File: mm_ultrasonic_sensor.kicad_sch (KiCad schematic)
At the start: 0 parts

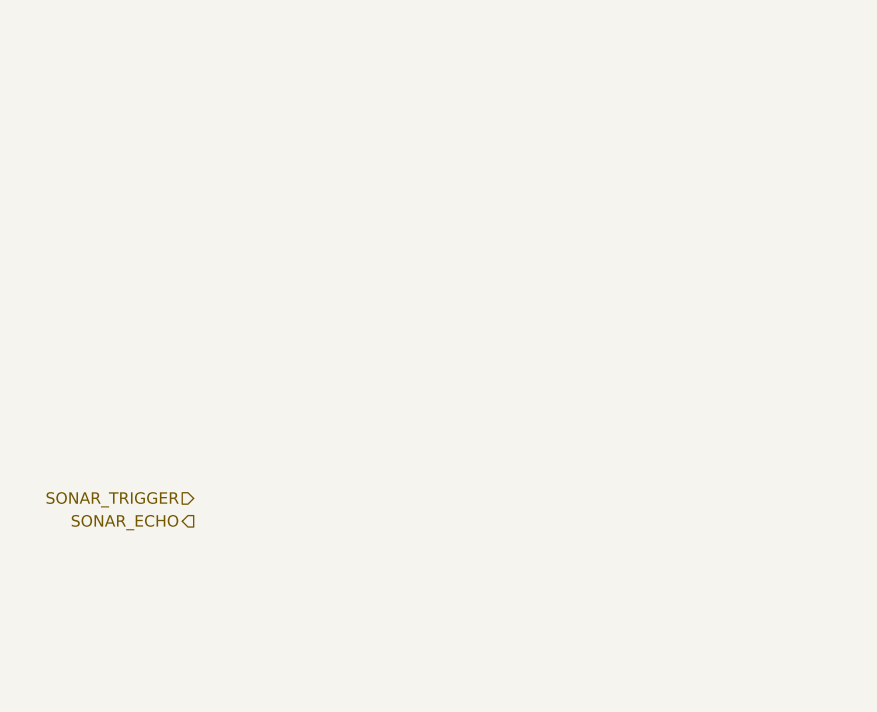
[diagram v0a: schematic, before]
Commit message: tp2
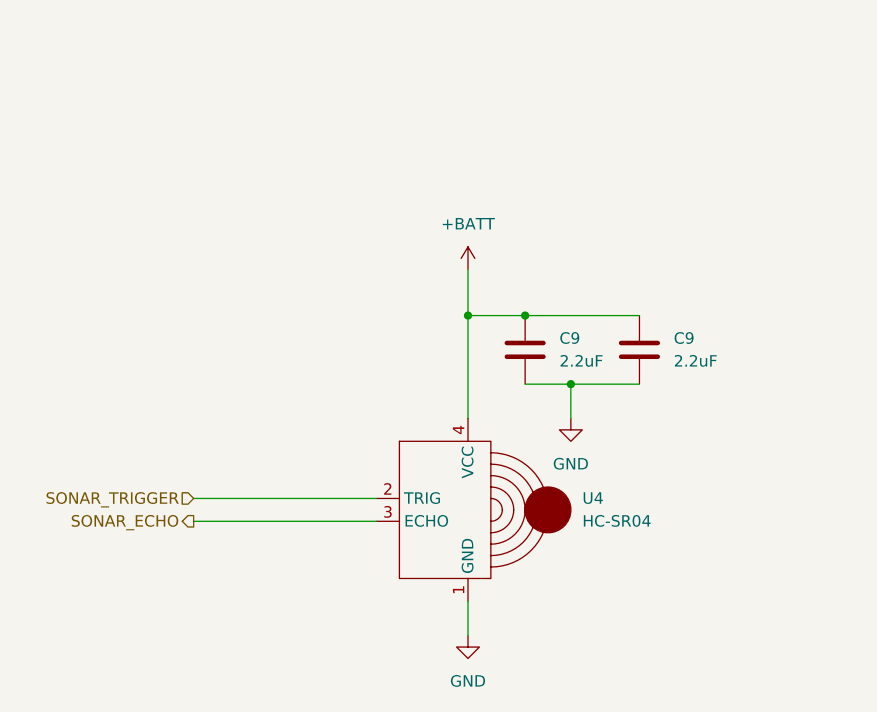
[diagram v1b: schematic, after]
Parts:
- added C9 (x2): 2.2uF, Capacitor_SMD:C_0603_1608Metric, symbol Device:C
- added U4: HC-SR04, minimouse:HC-SR04, symbol minimouse:HC-SR04
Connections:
- net SONAR_ECHO: now also U4.3 (ECHO)
- net SONAR_TRIGGER: now also U4.2 (TRIG)
- new net +BATT: C9.1, C9.1, U4.4 (VCC)
- new net GND: C9.2, C9.2, U4.1 (GND)
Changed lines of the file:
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@@
 (kicad_sch (version 20230121) (generator eeschema)
   (paper "A4")
+  (junction (at 139.7 68.58) (diameter 0) (color 0 0 0 0)
+  )
+  (junction (at 151.13 76.2) (diameter 0) (color 0 0 0 0)
+  )
+  (junction (at 146.05 68.58) (diameter 0) (color 0 0 0 0)
+  )
+  (wire (pts (xy 151.13 76.2) (xy 151.13 80.01))
+    (stroke (width 0) (type default))
+  )
+  (wire (pts (xy 151.13 76.2) (xy 158.75 76.2))
+    (stroke (width 0) (type default))
+  )
+  (wire (pts (xy 139.7 68.58) (xy 146.05 68.58))
+    (stroke (width 0) (type default))
+  )
+  (wire (pts (xy 146.05 76.2) (xy 151.13 76.2))
+    (stroke (width 0) (type default))
+  )
+  (wire (pts (xy 109.22 88.9) (xy 129.54 88.9))
+    (stroke (width 0) (type default))
+  )
+  (wire (pts (xy 139.7 100.33) (xy 139.7 104.14))
+    (stroke (width 0) (type default))
+  )
+  (wire (pts (xy 146.05 68.58) (xy 158.75 68.58))
+    (stroke (width 0) (type default))
+  )
+  (wire (pts (xy 139.7 68.58) (xy 139.7 80.01))
+    (stroke (width 0) (type default))
+  )
+  (wire (pts (xy 139.7 63.5) (xy 139.7 68.58))
+    (stroke (width 0) (type default))
+  )
+  (wire (pts (xy 109.22 91.44) (xy 129.54 91.44))
+    (stroke (width 0) (type default))
+  )
   (hierarchical_label "SONAR_TRIGGER" (shape input) (at 109.22 88.9 180) (fields_autoplaced)
     (effects (font (size 1.27 1.27)) (justify right))
@@
     (effects (font (size 1.27 1.27)) (justify right))
   )
+  (symbol (lib_id "power:GND") (at 151.13 80.01 0) (unit 1)
+    (in_bom yes) (on_board yes) (dnp no) (fields_autoplaced)
+    (property "Reference" "#PWR040" (at 151.13 86.36 0)
+      (effects (font (size 1.27 1.27)) hide)
+    )
+    (property "Value" "GND" (at 151.13 85.09 0)
+      (effects (font (size 1.27 1.27)))
+    )
+    (property "Footprint" "" (at 151.13 80.01 0)
+      (effects (font (size 1.27 1.27)) hide)
+    )
+    (property "Datasheet" "" (at 151.13 80.01 0)
+      (effects (font (size 1.27 1.27)) hide)
+    )
+    (pin "1")
+    (instances
+      (project "minimouse"
+        (path "/d8fa4cba-2469-4231-847f-065b6b829f44/224298a9-7d6e-4a70-a0a5-f2614895ec28"
+          (reference "#PWR040") (unit 1)
+        )
+      )
+    )
+  )
+  (symbol (lib_id "Device:C") (at 158.75 72.39 0) (unit 1)
+    (in_bom yes) (on_board yes) (dnp no) (fields_autoplaced)
+    (property "Reference" "C9" (at 162.56 71.12 0)
+      (effects (font (size 1.27 1.27)) (justify left))
+    )
+    (property "Value" "2.2uF" (at 162.56 73.66 0)
+      (effects (font (size 1.27 1.27)) (justify left))
+    )
+    (property "Footprint" "Capacitor_SMD:C_0603_1608Metric" (at 159.7152 76.2 0)
+      (effects (font (size 1.27 1.27)) hide)
+    )
+    (property "Datasheet" "~" (at 158.75 72.39 0)
+      (effects (font (size 1.27 1.27)) hide)
+    )
+    (pin "1")
+    (pin "2")
+    (instances
+      (project "minimouse"
+        (path "/d8fa4cba-2469-4231-847f-065b6b829f44/d17bb1c7-f68a-465e-9a17-5858ef86fc30"
+          (reference "C9") (unit 1)
+        )
+        (path "/d8fa4cba-2469-4231-847f-065b6b829f44/224298a9-7d6e-4a70-a0a5-f2614895ec28"
+          (reference "C16") (unit 1)
+        )
+      )
+    )
+  )
+  (symbol (lib_id "minimouse:HC-SR04") (at 139.7 90.17 0) (unit 1)
+    (in_bom yes) (on_board yes) (dnp no) (fields_autoplaced)
+    (property "Reference" "U4" (at 152.4 88.9 0)
+      (effects (font (size 1.27 1.27)) (justify left))
+    )
+    (property "Value" "HC-SR04" (at 152.4 91.44 0)
+      (effects (font (size 1.27 1.27)) (justify left))
+    )
+    (property "Footprint" "minimouse:HC-SR04" (at 139.7 90.17 0)
+      (effects (font (size 1.27 1.27)) hide)
+    )
+    (property "Datasheet" "" (at 139.7 90.17 0)
+      (effects (font (size 1.27 1.27)) hide)
+    )
+    (pin "2")
+    (pin "3")
+    (pin "4")
+    (pin "1")
+    (instances
+      (project "minimouse"
+        (path "/d8fa4cba-2469-4231-847f-065b6b829f44/224298a9-7d6e-4a70-a0a5-f2614895ec28"
+          (reference "U4") (unit 1)
+        )
+      )
+    )
+  )
+  (symbol (lib_id "power:+BATT") (at 139.7 63.5 0) (unit 1)
+    (in_bom yes) (on_board yes) (dnp no) (fields_autoplaced)
+    (property "Reference" "#PWR033" (at 139.7 67.31 0)
+      (effects (font (size 1.27 1.27)) hide)
+    )
+    (property "Value" "+BATT" (at 139.7 58.42 0)
+      (effects (font (size 1.27 1.27)))
+    )
+    (property "Footprint" "" (at 139.7 63.5 0)
+      (effects (font (size 1.27 1.27)) hide)
+    )
+    (property "Datasheet" "" (at 139.7 63.5 0)
+      (effects (font (size 1.27 1.27)) hide)
+    )
+    (pin "1")
+    (instances
+      (project "minimouse"
+        (path "/d8fa4cba-2469-4231-847f-065b6b829f44/224298a9-7d6e-4a70-a0a5-f2614895ec28"
+          (reference "#PWR033") (unit 1)
+        )
+      )
+    )
+  )
+  (symbol (lib_id "power:GND") (at 139.7 104.14 0) (unit 1)
+    (in_bom yes) (on_board yes) (dnp no) (fields_autoplaced)
+    (property "Reference" "#PWR032" (at 139.7 110.49 0)
+      (effects (font (size 1.27 1.27)) hide)
+    )
+    (property "Value" "GND" (at 139.7 109.22 0)
+      (effects (font (size 1.27 1.27)))
+    )
+    (property "Footprint" "" (at 139.7 104.14 0)
+      (effects (font (size 1.27 1.27)) hide)
+    )
+    (property "Datasheet" "" (at 139.7 104.14 0)
+      (effects (font (size 1.27 1.27)) hide)
+    )
+    (pin "1")
+    (instances
+      (project "minimouse"
+        (path "/d8fa4cba-2469-4231-847f-065b6b829f44/224298a9-7d6e-4a70-a0a5-f2614895ec28"
+          (reference "#PWR032") (unit 1)
+        )
+      )
+    )
+  )
+  (symbol (lib_id "Device:C") (at 146.05 72.39 0) (unit 1)
+    (in_bom yes) (on_board yes) (dnp no) (fields_autoplaced)
+    (property "Reference" "C9" (at 149.86 71.12 0)
+      (effects (font (size 1.27 1.27)) (justify left))
+    )
+    (property "Value" "2.2uF" (at 149.86 73.66 0)
+      (effects (font (size 1.27 1.27)) (justify left))
+    )
+    (property "Footprint" "Capacitor_SMD:C_0603_1608Metric" (at 147.0152 76.2 0)
+      (effects (font (size 1.27 1.27)) hide)
+    )
+    (property "Datasheet" "~" (at 146.05 72.39 0)
+      (effects (font (size 1.27 1.27)) hide)
+    )
+    (pin "1")
+    (pin "2")
+    (instances
+      (project "minimouse"
+        (path "/d8fa4cba-2469-4231-847f-065b6b829f44/d17bb1c7-f68a-465e-9a17-5858ef86fc30"
+          (reference "C9") (unit 1)
+        )
+        (path "/d8fa4cba-2469-4231-847f-065b6b829f44/224298a9-7d6e-4a70-a0a5-f2614895ec28"
+          (reference "C15") (unit 1)
+        )
+      )
+    )
+  )
 )

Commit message: TP3
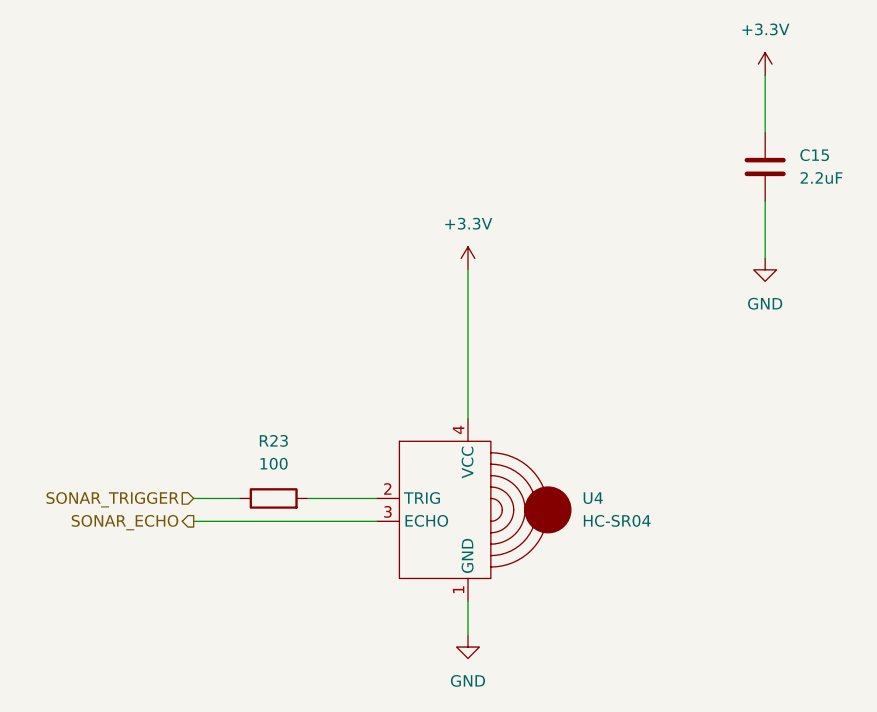
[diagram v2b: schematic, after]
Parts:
- removed C9 (x2): 2.2uF, Capacitor_SMD:C_0603_1608Metric, symbol Device:C
- added C15: 2.2uF, Capacitor_SMD:C_0603_1608Metric, symbol Device:C
- added R23: 100, Resistor_SMD:R_0603_1608Metric, symbol Device:R
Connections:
- net GND: now also C15.2
- net SONAR_TRIGGER: now also R23.1; no longer U4.2 (TRIG)
- net +BATT renamed +3.3V
- net +3.3V: now also C15.1
- new net: R23.2, U4.2 (TRIG)
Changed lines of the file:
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@@
 (kicad_sch (version 20230121) (generator eeschema)
   (paper "A4")
-  (junction (at 139.7 68.58) (diameter 0) (color 0 0 0 0)
-  )
-  (junction (at 151.13 76.2) (diameter 0) (color 0 0 0 0)
-  )
-  (junction (at 146.05 68.58) (diameter 0) (color 0 0 0 0)
-  )
-  (wire (pts (xy 151.13 76.2) (xy 151.13 80.01))
+  (wire (pts (xy 109.22 88.9) (xy 114.3 88.9))
     (stroke (width 0) (type default))
   )
-  (wire (pts (xy 151.13 76.2) (xy 158.75 76.2))
-    (stroke (width 0) (type default))
-  )
-  (wire (pts (xy 139.7 68.58) (xy 146.05 68.58))
-    (stroke (width 0) (type default))
-  )
-  (wire (pts (xy 146.05 76.2) (xy 151.13 76.2))
-    (stroke (width 0) (type default))
-  )
-  (wire (pts (xy 109.22 88.9) (xy 129.54 88.9))
+  (wire (pts (xy 172.72 41.91) (xy 172.72 48.26))
     (stroke (width 0) (type default))
   )
@@
     (stroke (width 0) (type default))
   )
-  (wire (pts (xy 146.05 68.58) (xy 158.75 68.58))
+  (wire (pts (xy 121.92 88.9) (xy 129.54 88.9))
     (stroke (width 0) (type default))
   )
-  (wire (pts (xy 139.7 68.58) (xy 139.7 80.01))
+  (wire (pts (xy 172.72 55.88) (xy 172.72 62.23))
     (stroke (width 0) (type default))
   )
-  (wire (pts (xy 139.7 63.5) (xy 139.7 68.58))
+  (wire (pts (xy 139.7 63.5) (xy 139.7 80.01))
     (stroke (width 0) (type default))
   )
@@
     (effects (font (size 1.27 1.27)) (justify right))
   )
-  (symbol (lib_id "power:GND") (at 151.13 80.01 0) (unit 1)
+  (symbol (lib_id "power:GND") (at 172.72 62.23 0) (unit 1)
     (in_bom yes) (on_board yes) (dnp no) (fields_autoplaced)
-    (property "Reference" "#PWR040" (at 151.13 86.36 0)
+    (property "Reference" "#PWR043" (at 172.72 68.58 0)
       (effects (font (size 1.27 1.27)) hide)
     )
-    (property "Value" "GND" (at 151.13 85.09 0)
+    (property "Value" "GND" (at 172.72 67.31 0)
       (effects (font (size 1.27 1.27)))
     )
-    (property "Footprint" "" (at 151.13 80.01 0)
+    (property "Footprint" "" (at 172.72 62.23 0)
       (effects (font (size 1.27 1.27)) hide)
     )
-    (property "Datasheet" "" (at 151.13 80.01 0)
+    (property "Datasheet" "" (at 172.72 62.23 0)
       (effects (font (size 1.27 1.27)) hide)
     )
@@
       (project "minimouse"
         (path "/d8fa4cba-2469-4231-847f-065b6b829f44/224298a9-7d6e-4a70-a0a5-f2614895ec28"
-          (reference "#PWR040") (unit 1)
-        )
-      )
-    )
-  )
-  (symbol (lib_id "Device:C") (at 158.75 72.39 0) (unit 1)
-    (in_bom yes) (on_board yes) (dnp no) (fields_autoplaced)
-    (property "Reference" "C9" (at 162.56 71.12 0)
-      (effects (font (size 1.27 1.27)) (justify left))
-    )
-    (property "Value" "2.2uF" (at 162.56 73.66 0)
-      (effects (font (size 1.27 1.27)) (justify left))
-    )
-    (property "Footprint" "Capacitor_SMD:C_0603_1608Metric" (at 159.7152 76.2 0)
-      (effects (font (size 1.27 1.27)) hide)
-    )
-    (property "Datasheet" "~" (at 158.75 72.39 0)
-      (effects (font (size 1.27 1.27)) hide)
-    )
-    (pin "1")
-    (pin "2")
-    (instances
-      (project "minimouse"
-        (path "/d8fa4cba-2469-4231-847f-065b6b829f44/d17bb1c7-f68a-465e-9a17-5858ef86fc30"
-          (reference "C9") (unit 1)
-        )
-        (path "/d8fa4cba-2469-4231-847f-065b6b829f44/224298a9-7d6e-4a70-a0a5-f2614895ec28"
-          (reference "C16") (unit 1)
+          (reference "#PWR043") (unit 1)
         )
       )
@@
     )
   )
-  (symbol (lib_id "power:+BATT") (at 139.7 63.5 0) (unit 1)
+  (symbol (lib_id "Device:C") (at 172.72 52.07 0) (unit 1)
     (in_bom yes) (on_board yes) (dnp no) (fields_autoplaced)
-    (property "Reference" "#PWR033" (at 139.7 67.31 0)
+    (property "Reference" "C15" (at 176.53 50.8 0)
+      (effects (font (size 1.27 1.27)) (justify left))
+    )
+    (property "Value" "2.2uF" (at 176.53 53.34 0)
+      (effects (font (size 1.27 1.27)) (justify left))
+    )
+    (property "Footprint" "Capacitor_SMD:C_0603_1608Metric" (at 173.6852 55.88 0)
       (effects (font (size 1.27 1.27)) hide)
     )
-    (property "Value" "+BATT" (at 139.7 58.42 0)
+    (property "Datasheet" "~" (at 172.72 52.07 0)
+      (effects (font (size 1.27 1.27)) hide)
+    )
+    (pin "1")
+    (pin "2")
+    (instances
+      (project "minimouse"
+        (path "/d8fa4cba-2469-4231-847f-065b6b829f44/224298a9-7d6e-4a70-a0a5-f2614895ec28"
+          (reference "C15") (unit 1)
+        )
+      )
+    )
+  )
+  (symbol (lib_id "Device:R") (at 118.11 88.9 90) (unit 1)
+    (in_bom yes) (on_board yes) (dnp no) (fields_autoplaced)
+    (property "Reference" "R23" (at 118.11 82.55 90)
       (effects (font (size 1.27 1.27)))
     )
-    (property "Footprint" "" (at 139.7 63.5 0)
+    (property "Value" "100" (at 118.11 85.09 90)
+      (effects (font (size 1.27 1.27)))
+    )
+    (property "Footprint" "Resistor_SMD:R_0603_1608Metric" (at 118.11 90.678 90)
       (effects (font (size 1.27 1.27)) hide)
     )
-    (property "Datasheet" "" (at 139.7 63.5 0)
+    (property "Datasheet" "~" (at 118.11 88.9 0)
       (effects (font (size 1.27 1.27)) hide)
     )
+    (pin "2")
     (pin "1")
     (instances
       (project "minimouse"
         (path "/d8fa4cba-2469-4231-847f-065b6b829f44/224298a9-7d6e-4a70-a0a5-f2614895ec28"
-          (reference "#PWR033") (unit 1)
+          (reference "R23") (unit 1)
         )
       )
@@
     )
   )
-  (symbol (lib_id "Device:C") (at 146.05 72.39 0) (unit 1)
+  (symbol (lib_id "power:+3.3V") (at 139.7 63.5 0) (unit 1)
     (in_bom yes) (on_board yes) (dnp no) (fields_autoplaced)
-    (property "Reference" "C9" (at 149.86 71.12 0)
-      (effects (font (size 1.27 1.27)) (justify left))
-    )
-    (property "Value" "2.2uF" (at 149.86 73.66 0)
-      (effects (font (size 1.27 1.27)) (justify left))
-    )
-    (property "Footprint" "Capacitor_SMD:C_0603_1608Metric" (at 147.0152 76.2 0)
+    (property "Reference" "#PWR033" (at 139.7 67.31 0)
       (effects (font (size 1.27 1.27)) hide)
     )
-    (property "Datasheet" "~" (at 146.05 72.39 0)
+    (property "Value" "+3.3V" (at 139.7 58.42 0)
+      (effects (font (size 1.27 1.27)))
+    )
+    (property "Footprint" "" (at 139.7 63.5 0)
+      (effects (font (size 1.27 1.27)) hide)
+    )
+    (property "Datasheet" "" (at 139.7 63.5 0)
       (effects (font (size 1.27 1.27)) hide)
     )
     (pin "1")
-    (pin "2")
     (instances
       (project "minimouse"
-        (path "/d8fa4cba-2469-4231-847f-065b6b829f44/d17bb1c7-f68a-465e-9a17-5858ef86fc30"
-          (reference "C9") (unit 1)
-        )
         (path "/d8fa4cba-2469-4231-847f-065b6b829f44/224298a9-7d6e-4a70-a0a5-f2614895ec28"
-          (reference "C15") (unit 1)
+          (reference "#PWR033") (unit 1)
         )
       )
+    )
+  )
+  (symbol (lib_id "power:+3.3V") (at 172.72 41.91 0) (unit 1)
+    (in_bom yes) (on_board yes) (dnp no) (fields_autoplaced)
+    (property "Reference" "#PWR035" (at 172.72 45.72 0)
+      (effects (font (size 1.27 1.27)) hide)
+    )
+    (property "Value" "+3.3V" (at 172.72 36.83 0)
+      (effects (font (size 1.27 1.27)))
+    )
+    (property "Footprint" "" (at 172.72 41.91 0)
+      (effects (font (size 1.27 1.27)) hide)
+    )
+    (property "Datasheet" "" (at 172.72 41.91 0)
+      (effects (font (size 1.27 1.27)) hide)
+    )
+    (pin "1")
+    (instances
+      (project "minimouse"
+        (path "/d8fa4cba-2469-4231-847f-065b6b829f44/224298a9-7d6e-4a70-a0a5-f2614895ec28"
+          (reference "#PWR035") (unit 1)
+        )
+      )
